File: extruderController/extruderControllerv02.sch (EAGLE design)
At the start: 72 parts, among them IC1 LM1117MPX-5.0, IC2 MAX3467CPA, IC3 ATMEGA2561-16AU, IC4 ULN2003AD, J1 RJ45, Q2 PH7030L, Q3 PH7030L, Q4 PH7030L, Q5 PH7030L, Q6 PH7030L, X1 22-23-2081, X2 22-23-2081, X3 22-23-2101, X6 22-23-2041, X8 22-23-2031, X9 22-23-2031

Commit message: c
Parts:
- added J4: (no value), SparkFun-Connectors:CONN_023.5MM
- Q1: SPICEPREFIX (none) -> B
- R10, R2, R4, R6, R8: value (none) -> 10
- R11, R3, R5, R7, R9: value (none) -> 100k
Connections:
- net +12V: now also J4.1
- net GND: now also J4.2
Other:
- note added: "I/O"
- moved on the sheet: C1, C10, C11, C12, C16, C17, C18, C2, C5, C6, C8, C9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

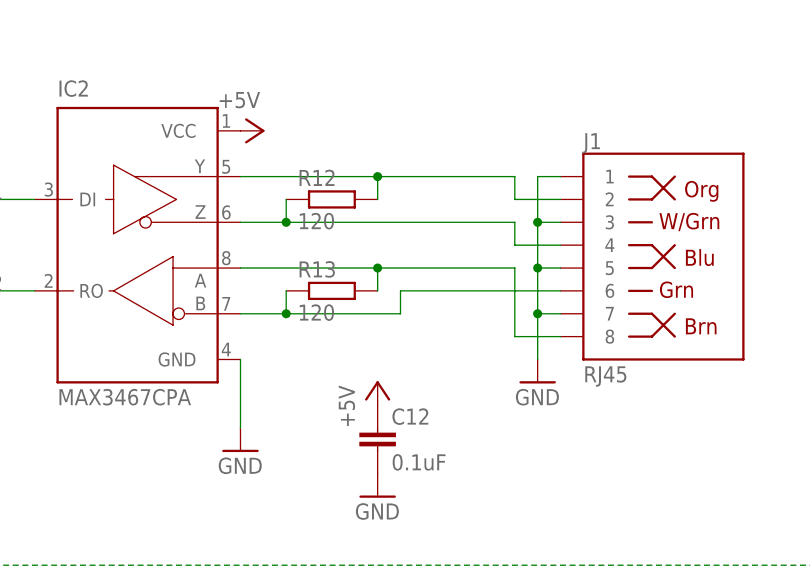
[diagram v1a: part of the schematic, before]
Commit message: c
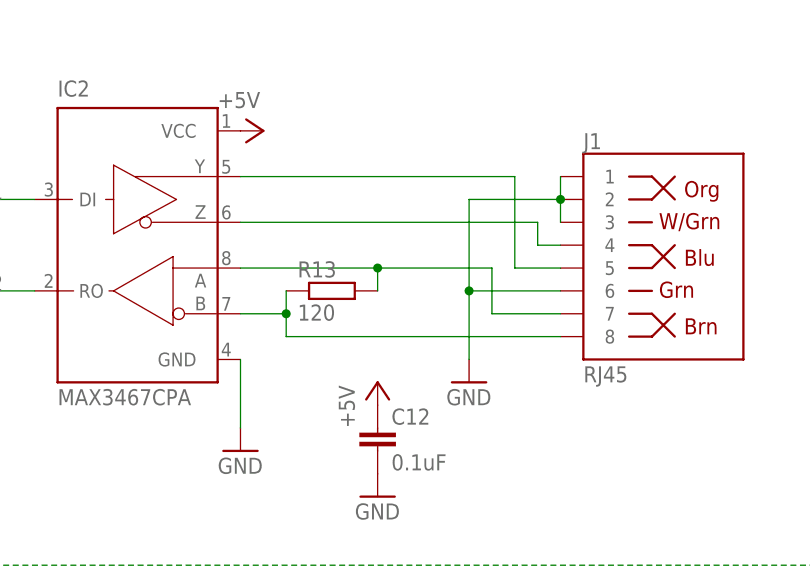
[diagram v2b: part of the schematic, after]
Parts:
- removed R12: 120, rcl:R-EU_R1210
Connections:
- removed net N$35: IC2.Y, J1.2, R12.2
- new net N$45: IC2.Z, J1.4
- net GND: now also J1.2, J1.6; no longer J1.5, J1.7
- net N$27: now also J1.8; no longer J1.6
- net N$33: now also IC2.Y, J1.5; no longer IC2.Z, J1.4, R12.1
- net N$36: now also J1.7; no longer J1.8
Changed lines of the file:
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@@
 <?xml version="1.0" encoding="utf-8"?>
 <!DOCTYPE eagle SYSTEM "eagle.dtd">
-<eagle version="9.2.2">
+<eagle version="9.3.1">
 <drawing>
 <settings>
@@
 <part name="GND21" library="supply1" library_urn="urn:adsk.eagle:library:371" deviceset="GND" device=""/>
 <part name="C12" library="rcl" library_urn="urn:adsk.eagle:library:334" deviceset="C-EU" device="C0603" package3d_urn="urn:adsk.eagle:package:23616/2" value="0.1uF"/>
-<part name="R12" library="rcl" library_urn="urn:adsk.eagle:library:334" deviceset="R-EU_" device="R1210" package3d_urn="urn:adsk.eagle:package:23554/2" value="120"/>
 <part name="R13" library="rcl" library_urn="urn:adsk.eagle:library:334" deviceset="R-EU_" device="R1210" package3d_urn="urn:adsk.eagle:package:23554/2" value="120"/>
 <part name="P+14" library="supply1" library_urn="urn:adsk.eagle:library:371" deviceset="+5V" device=""/>
@@
 <attribute name="VALUE" x="118.364" y="165.481" size="1.778" layer="96"/>
 </instance>
-<instance part="R12" gate="G$1" x="111.76" y="195.58" smashed="yes">
-<attribute name="NAME" x="107.95" y="197.0786" size="1.778" layer="95"/>
-<attribute name="VALUE" x="107.95" y="192.278" size="1.778" layer="96"/>
-</instance>
 <instance part="R13" gate="G$1" x="111.76" y="185.42" smashed="yes">
 <attribute name="NAME" x="107.95" y="186.9186" size="1.778" layer="95"/>
@@
 <attribute name="VALUE" x="114.3" y="160.02" size="1.778" layer="96"/>
 </instance>
-<instance part="GND24" gate="1" x="134.62" y="175.26" smashed="yes">
-<attribute name="VALUE" x="132.08" y="172.72" size="1.778" layer="96"/>
+<instance part="GND24" gate="1" x="127" y="175.26" smashed="yes">
+<attribute name="VALUE" x="124.46" y="172.72" size="1.778" layer="96"/>
 </instance>
 <instance part="X8" gate="-1" x="109.22" y="12.7" smashed="yes" rot="R180">
@@
 <pinref part="R18" gate="G$1" pin="1"/>
 <pinref part="GND25" gate="1" pin="GND"/>
-</segment>
-<segment>
-<pinref part="J1" gate="JP1" pin="1"/>
-<wire x1="137.16" y1="198.12" x2="134.62" y2="198.12" width="0.1524" layer="91"/>
-<wire x1="134.62" y1="198.12" x2="134.62" y2="193.04" width="0.1524" layer="91"/>
-<pinref part="J1" gate="JP1" pin="3"/>
-<wire x1="134.62" y1="193.04" x2="137.16" y2="193.04" width="0.1524" layer="91"/>
-<wire x1="134.62" y1="193.04" x2="134.62" y2="187.96" width="0.1524" layer="91"/>
-<junction x="134.62" y="193.04"/>
-<pinref part="J1" gate="JP1" pin="5"/>
-<wire x1="134.62" y1="187.96" x2="137.16" y2="187.96" width="0.1524" layer="91"/>
-<wire x1="134.62" y1="187.96" x2="134.62" y2="182.88" width="0.1524" layer="91"/>
-<junction x="134.62" y="187.96"/>
-<pinref part="J1" gate="JP1" pin="7"/>
-<wire x1="134.62" y1="182.88" x2="137.16" y2="182.88" width="0.1524" layer="91"/>
-<pinref part="GND24" gate="1" pin="GND"/>
-<wire x1="134.62" y1="182.88" x2="134.62" y2="177.8" width="0.1524" layer="91"/>
-<junction x="134.62" y="182.88"/>
 </segment>
 <segment>
@@
 <pinref part="GND31" gate="1" pin="GND"/>
 <wire x1="-93.98" y1="203.2" x2="-93.98" y2="205.74" width="0.1524" layer="91"/>
+</segment>
+<segment>
+<pinref part="J1" gate="JP1" pin="1"/>
+<pinref part="J1" gate="JP1" pin="2"/>
+<wire x1="137.16" y1="198.12" x2="137.16" y2="195.58" width="0.1524" layer="91"/>
+<pinref part="J1" gate="JP1" pin="3"/>
+<wire x1="137.16" y1="193.04" x2="137.16" y2="195.58" width="0.1524" layer="91"/>
+<junction x="137.16" y="195.58"/>
+<wire x1="137.16" y1="195.58" x2="127" y2="195.58" width="0.1524" layer="91"/>
+<wire x1="127" y1="195.58" x2="127" y2="185.42" width="0.1524" layer="91"/>
+<pinref part="J1" gate="JP1" pin="6"/>
+<wire x1="127" y1="185.42" x2="137.16" y2="185.42" width="0.1524" layer="91"/>
+<wire x1="127" y1="185.42" x2="127" y2="177.8" width="0.1524" layer="91"/>
+<junction x="127" y="185.42"/>
+<pinref part="GND24" gate="1" pin="GND"/>
 </segment>
 </net>
@@
 <wire x1="106.68" y1="182.88" x2="101.6" y2="182.88" width="0.1524" layer="91"/>
 <wire x1="106.68" y1="185.42" x2="106.68" y2="182.88" width="0.1524" layer="91"/>
-<pinref part="J1" gate="JP1" pin="6"/>
-<wire x1="137.16" y1="185.42" x2="119.38" y2="185.42" width="0.1524" layer="91"/>
-<wire x1="119.38" y1="185.42" x2="119.38" y2="182.88" width="0.1524" layer="91"/>
-<wire x1="119.38" y1="182.88" x2="106.68" y2="182.88" width="0.1524" layer="91"/>
+<pinref part="J1" gate="JP1" pin="8"/>
+<wire x1="137.16" y1="180.34" x2="106.68" y2="180.34" width="0.1524" layer="91"/>
+<wire x1="106.68" y1="180.34" x2="106.68" y2="182.88" width="0.1524" layer="91"/>
 <junction x="106.68" y="182.88"/>
-</segment>
-</net>
-<net name="N$33" class="0">
-<segment>
-<pinref part="IC2" gate="G$1" pin="Z"/>
-<wire x1="101.6" y1="193.04" x2="106.68" y2="193.04" width="0.1524" layer="91"/>
-<pinref part="R12" gate="G$1" pin="1"/>
-<wire x1="106.68" y1="195.58" x2="106.68" y2="193.04" width="0.1524" layer="91"/>
-<wire x1="106.68" y1="193.04" x2="132.08" y2="193.04" width="0.1524" layer="91"/>
-<junction x="106.68" y="193.04"/>
-<wire x1="132.08" y1="193.04" x2="132.08" y2="190.5" width="0.1524" layer="91"/>
-<pinref part="J1" gate="JP1" pin="4"/>
-<wire x1="132.08" y1="190.5" x2="137.16" y2="190.5" width="0.1524" layer="91"/>
-</segment>
-</net>
-<net name="N$35" class="0">
-<segment>
-<pinref part="IC2" gate="G$1" pin="Y"/>
-<wire x1="101.6" y1="198.12" x2="116.84" y2="198.12" width="0.1524" layer="91"/>
-<pinref part="R12" gate="G$1" pin="2"/>
-<wire x1="116.84" y1="195.58" x2="116.84" y2="198.12" width="0.1524" layer="91"/>
-<wire x1="116.84" y1="198.12" x2="132.08" y2="198.12" width="0.1524" layer="91"/>
-<wire x1="132.08" y1="198.12" x2="132.08" y2="195.58" width="0.1524" layer="91"/>
-<junction x="116.84" y="198.12"/>
-<pinref part="J1" gate="JP1" pin="2"/>
-<wire x1="132.08" y1="195.58" x2="137.16" y2="195.58" width="0.1524" layer="91"/>
 </segment>
 </net>
@@
 <pinref part="R13" gate="G$1" pin="2"/>
 <wire x1="116.84" y1="185.42" x2="116.84" y2="187.96" width="0.1524" layer="91"/>
-<wire x1="116.84" y1="187.96" x2="132.08" y2="187.96" width="0.1524" layer="91"/>
+<wire x1="116.84" y1="187.96" x2="129.54" y2="187.96" width="0.1524" layer="91"/>
 <junction x="116.84" y="187.96"/>
-<wire x1="132.08" y1="187.96" x2="132.08" y2="180.34" width="0.1524" layer="91"/>
-<pinref part="J1" gate="JP1" pin="8"/>
-<wire x1="132.08" y1="180.34" x2="137.16" y2="180.34" width="0.1524" layer="91"/>
+<wire x1="129.54" y1="187.96" x2="129.54" y2="182.88" width="0.1524" layer="91"/>
+<pinref part="J1" gate="JP1" pin="7"/>
+<wire x1="129.54" y1="182.88" x2="137.16" y2="182.88" width="0.1524" layer="91"/>
 </segment>
 </net>
@@
 </segment>
 </net>
+<net name="N$45" class="0">
+<segment>
+<pinref part="IC2" gate="G$1" pin="Z"/>
+<wire x1="101.6" y1="193.04" x2="134.62" y2="193.04" width="0.1524" layer="91"/>
+<pinref part="J1" gate="JP1" pin="4"/>
+<wire x1="137.16" y1="190.5" x2="134.62" y2="190.5" width="0.1524" layer="91"/>
+<wire x1="134.62" y1="190.5" x2="134.62" y2="193.04" width="0.1524" layer="91"/>
+</segment>
+</net>
+<net name="N$33" class="0">
+<segment>
+<pinref part="J1" gate="JP1" pin="5"/>
+<wire x1="137.16" y1="187.96" x2="132.08" y2="187.96" width="0.1524" layer="91"/>
+<pinref part="IC2" gate="G$1" pin="Y"/>
+<wire x1="101.6" y1="198.12" x2="132.08" y2="198.12" width="0.1524" layer="91"/>
+<wire x1="132.08" y1="187.96" x2="132.08" y2="198.12" width="0.1524" layer="91"/>
+</segment>
+</net>

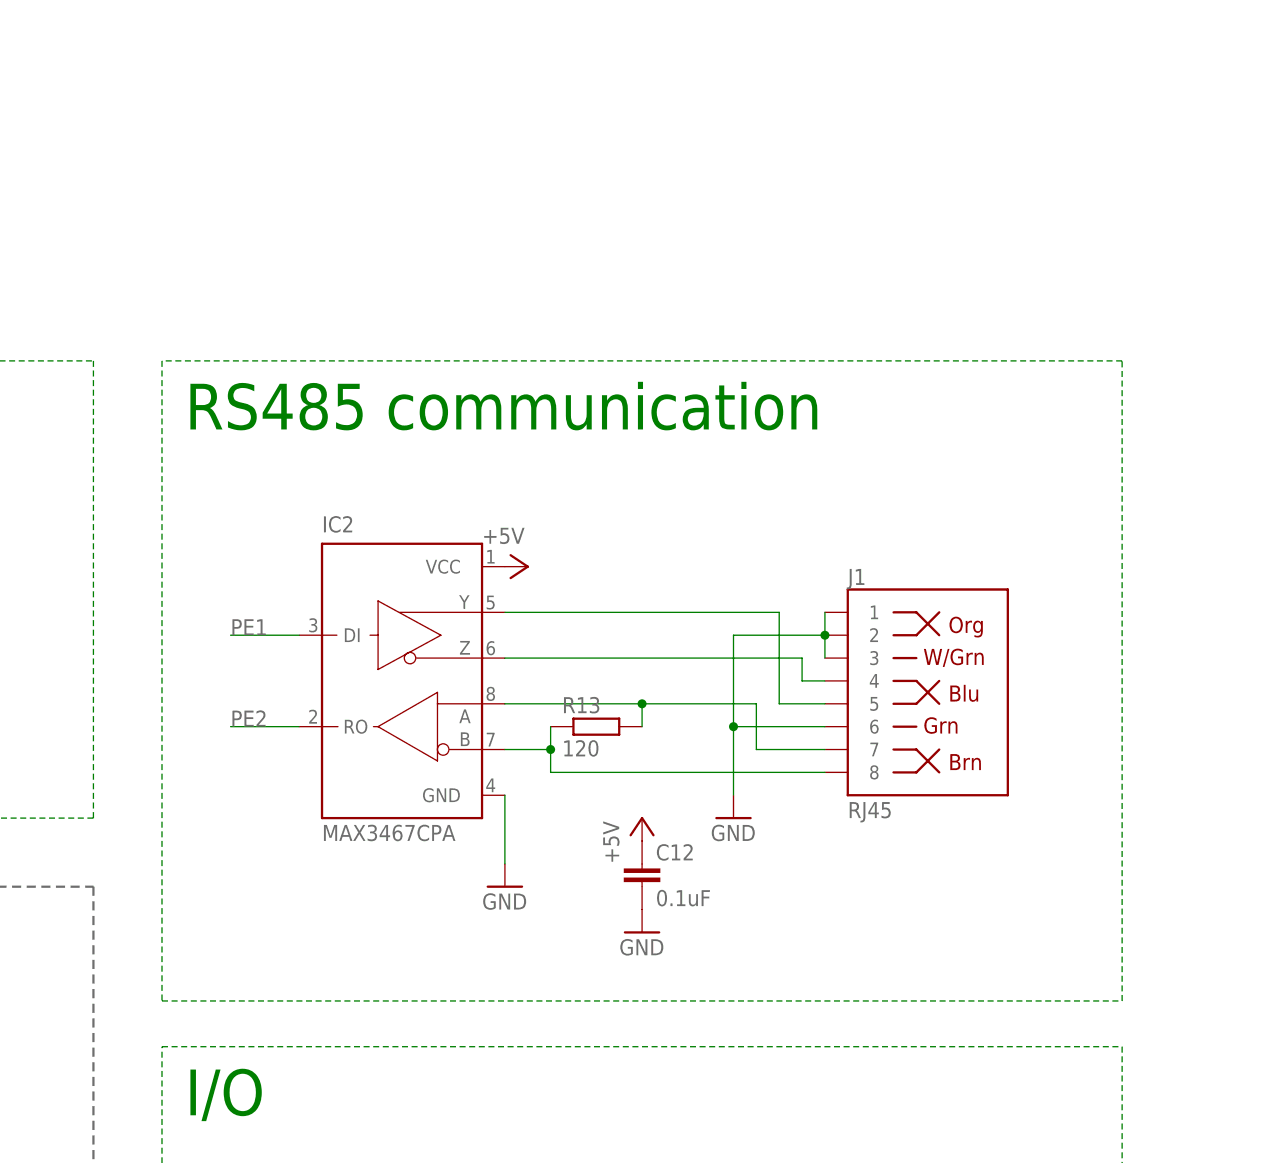
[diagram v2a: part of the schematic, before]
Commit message: f
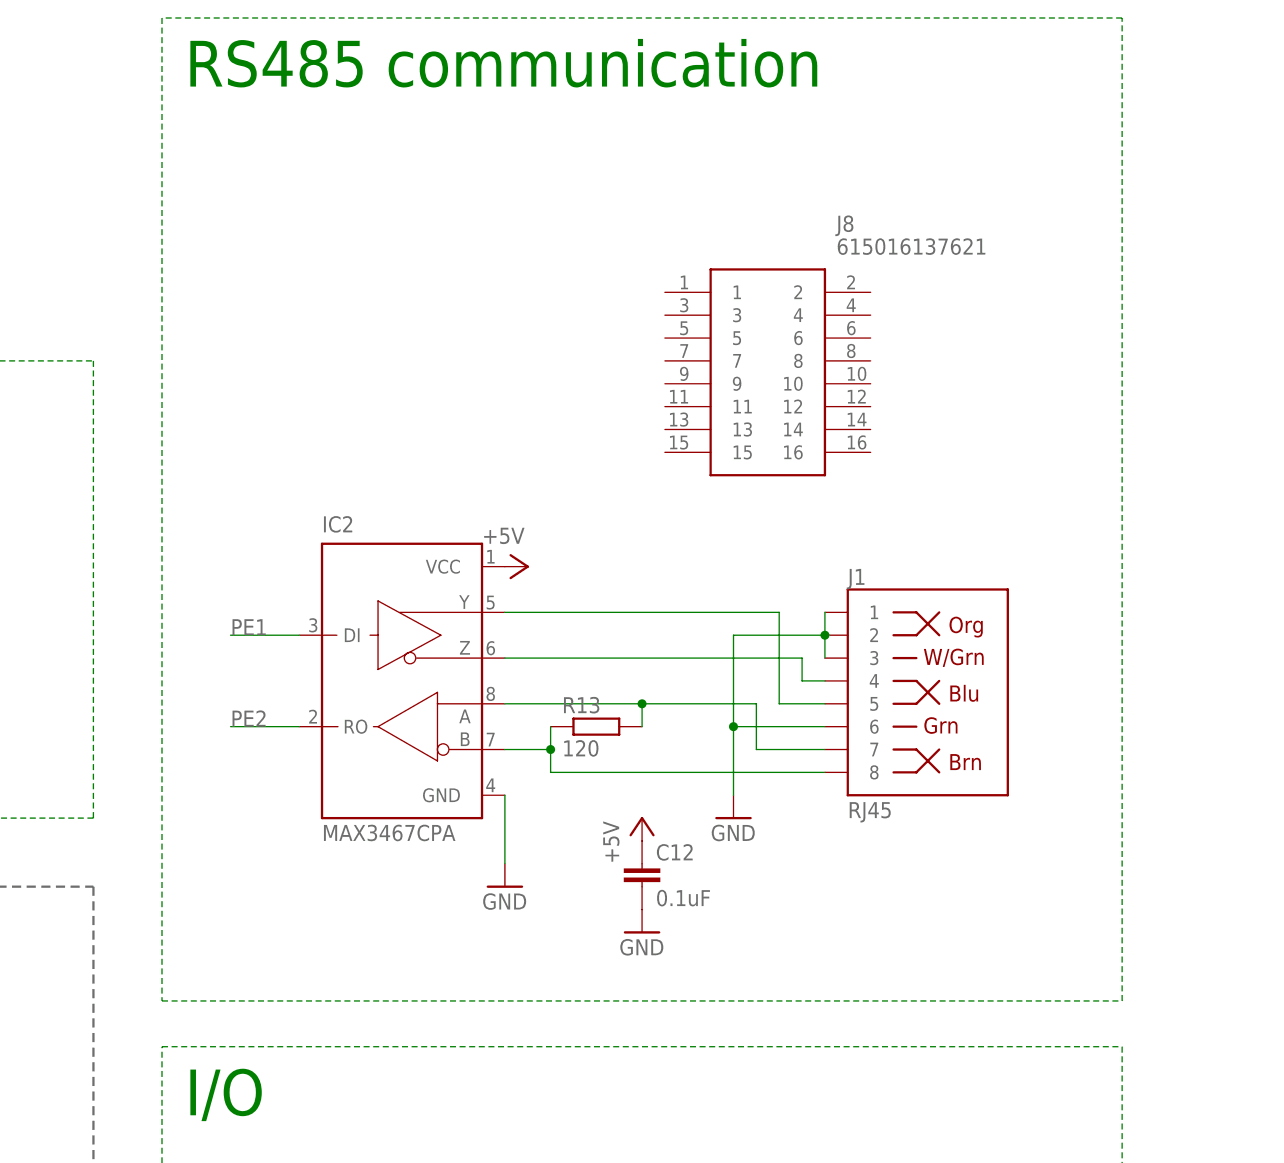
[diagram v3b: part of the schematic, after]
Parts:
- added J8: 615016137621, SamacSys_Parts:615016137621
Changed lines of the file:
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@@
 <?xml version="1.0" encoding="utf-8"?>
 <!DOCTYPE eagle SYSTEM "eagle.dtd">
-<eagle version="9.3.1">
+<eagle version="9.2.2">
 <drawing>
 <settings>
@@
 <part name="P+28" library="supply1" library_urn="urn:adsk.eagle:library:371" deviceset="+12V" device=""/>
 <part name="GND31" library="supply1" library_urn="urn:adsk.eagle:library:371" deviceset="GND" device=""/>
+<part name="J8" library="SamacSys_Parts" deviceset="615016137621" device=""/>
 </parts>
 <sheets>
@@
 <text x="-243.84" y="210.82" size="5.08" layer="91">Main stepper control output</text>
 <text x="66.04" y="76.2" size="5.08" layer="91">Hall effect sensor (rpm) input</text>
-<text x="66.04" y="218.44" size="5.08" layer="91">RS485 communication</text>
+<text x="66.04" y="256.54" size="5.08" layer="91">RS485 communication</text>
 <text x="66.04" y="27.94" size="5.08" layer="91">Hopper level sensor input</text>
 <wire x1="-109.22" y1="167.64" x2="55.88" y2="167.64" width="0.254" layer="95" style="longdash"/>
@@
 <instance part="GND31" gate="1" x="-93.98" y="200.66" smashed="yes">
 <attribute name="VALUE" x="-96.52" y="198.12" size="1.778" layer="96"/>
+</instance>
+<instance part="J8" gate="G$1" x="119.38" y="233.68" smashed="yes">
+<attribute name="NAME" x="138.43" y="241.3" size="1.778" layer="95" align="center-left"/>
+<attribute name="VALUE" x="138.43" y="238.76" size="1.778" layer="96" align="center-left"/>
 </instance>
 </instances>
@@
 <net name="N$42" class="0">
 <segment>
-<wire x1="63.5" y1="226.06" x2="63.5" y2="154.94" width="0.1524" layer="91" style="longdash"/>
+<wire x1="63.5" y1="264.16" x2="63.5" y2="154.94" width="0.1524" layer="91" style="longdash"/>
 <wire x1="63.5" y1="154.94" x2="170.18" y2="154.94" width="0.1524" layer="91" style="longdash"/>
-<wire x1="170.18" y1="154.94" x2="170.18" y2="226.06" width="0.1524" layer="91" style="longdash"/>
-<wire x1="170.18" y1="226.06" x2="63.5" y2="226.06" width="0.1524" layer="91" style="longdash"/>
-</segment>
-</net>
+<wire x1="170.18" y1="154.94" x2="170.18" y2="264.16" width="0.1524" layer="91" style="longdash"/>
+<wire x1="170.18" y1="264.16" x2="63.5" y2="264.16" width="0.1524" layer="91" style="longdash"/>
+</segment>
+</net>
